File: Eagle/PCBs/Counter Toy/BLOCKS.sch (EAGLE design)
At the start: 6 parts, among them U1 MC74HC1G14DTT1G

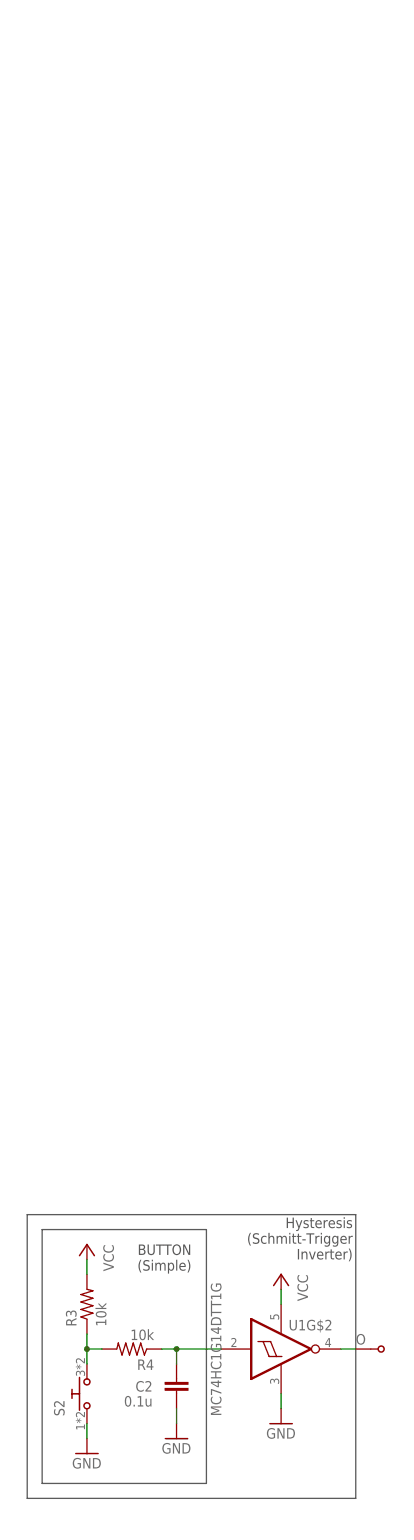
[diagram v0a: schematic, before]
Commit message: Better DFF
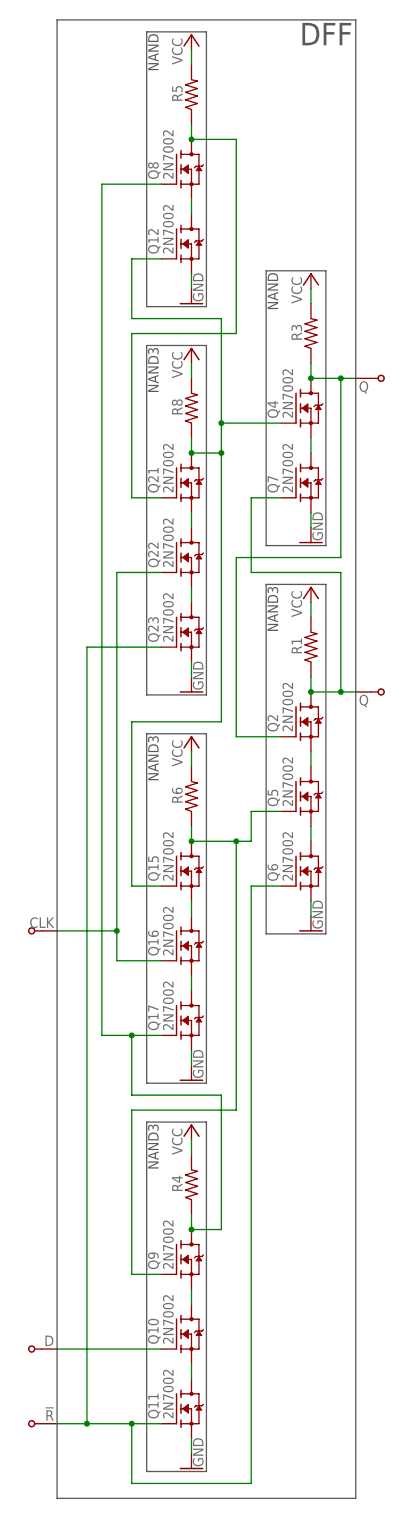
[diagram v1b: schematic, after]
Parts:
- removed C2: 0.1u, ellajameson-core:CAP0603
- removed O: TPPAD6, ellajameson-core:TPPAD6
- removed S2: (no value), ellajameson-core:SWITCH-NO-MOMPTS815SJM250SMTRLFS
- removed U1: MC74HC1G14DTT1G, ellajameson-core:MC74HC1G14DTT1G
- added !Q, !R, CLK, D, Q: TPPAD6, ellajameson-core:TPPAD6
- added Q10, Q11, Q12, Q15, Q16, Q17, Q2, Q21, Q22, Q23, Q4, Q5, Q6, Q7, Q8, Q9: 2N7002, ellajameson-core:2N7002
- added R1, R5, R6, R8: (no value), ellajameson-core:RES0603
- R3, R4: value 10k -> (none)
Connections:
- removed net N$1: O.S, U1G$2.O
- removed net N$3: R3.1, R4.2, S2.S
- new net N$10: Q2.S, Q5.D
- new net N$12: Q5.S, Q6.D
- new net N$14: Q4.S, Q7.D
- new net N$16: Q21.G, Q8.D, R5.1
- new net N$18: Q17.G, Q8.G, Q9.D, R4.1
- new net N$19: D.S, Q10.G
- new net N$20: Q10.D, Q9.S
- new net N$22: Q10.S, Q11.D
- new net N$24: Q12.D, Q8.S
- new net N$31: CLK.S, Q16.G, Q22.G
- new net N$32: Q15.S, Q16.D
- new net N$34: Q16.S, Q17.D
- new net N$44: Q21.S, Q22.D
- new net N$45: !R.S, Q11.G, Q23.G, Q6.G
- new net N$46: Q22.S, Q23.D
- new net N$7: Q12.G, Q15.G, Q21.D, Q4.G, R8.1
- new net N$8: Q.S, Q2.G, Q4.D, R3.1
- new net N$9: Q15.D, Q5.G, Q9.G, R6.1
- net GND: now also Q11.S, Q12.S, Q17.S, Q23.S, Q6.S, Q7.S; no longer C2.2, S2.P, U1G$1.V-
- net N$4: now also !Q.S, Q2.D, Q7.G, R1.1; no longer C2.1, R4.1, U1G$2.I
- net VCC: now also R1.2, R4.2, R5.2, R6.2, R8.2; no longer U1G$1.V+
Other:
- note added: "DFF"
- note added: "NAND"
- note added: "NAND3"
- note removed: "BUTTON (Simple)"
- note removed: "Hysteresis (Schmitt-Trigger Inverter)"
- moved on the sheet: R3, R4

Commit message: Testing open collector setup
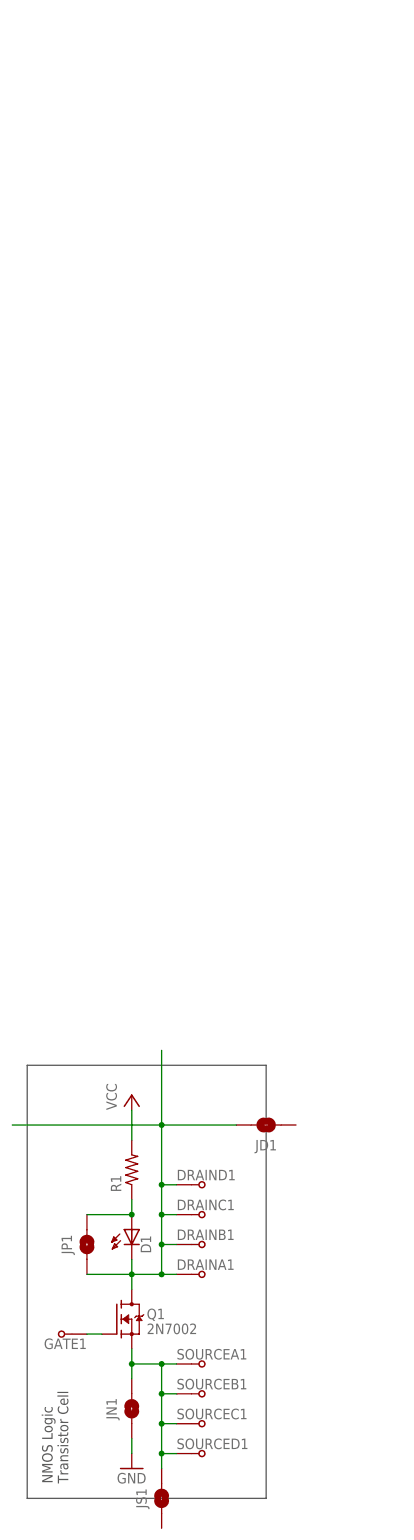
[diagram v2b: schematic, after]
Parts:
- removed !Q, !R, CLK, D, Q: TPPAD6, ellajameson-core:TPPAD6
- removed Q10, Q11, Q12, Q15, Q16, Q17, Q2, Q21, Q22, Q23, Q4, Q5, Q6, Q7, Q8, Q9: 2N7002, ellajameson-core:2N7002
- removed R3, R4, R5, R6, R8: (no value), ellajameson-core:RES0603
- added D1: (no value), ellajameson-core:LED0603
- added DRAINA1, DRAINB1, DRAINC1, DRAIND1, GATE1, SOURCEA1, SOURCEB1, SOURCEC1, SOURCED1: TPWIRE, ellajameson-core:TPWIRE
- added JD1, JN1, JP1, JS1: SJ_NO, ellajameson-core:SJ_NO
- added Q1: 2N7002, ellajameson-core:2N7002
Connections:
- removed net N$10: Q2.S, Q5.D
- removed net N$12: Q5.S, Q6.D
- removed net N$14: Q4.S, Q7.D
- removed net N$16: Q21.G, Q8.D, R5.1
- removed net N$18: Q17.G, Q8.G, Q9.D, R4.1
- removed net N$19: D.S, Q10.G
- removed net N$20: Q10.D, Q9.S
- removed net N$22: Q10.S, Q11.D
- removed net N$24: Q12.D, Q8.S
- removed net N$31: CLK.S, Q16.G, Q22.G
- removed net N$32: Q15.S, Q16.D
- removed net N$34: Q16.S, Q17.D
- removed net N$4: !Q.S, Q2.D, Q7.G, R1.1
- removed net N$44: Q21.S, Q22.D
- removed net N$45: !R.S, Q11.G, Q23.G, Q6.G
- removed net N$46: Q22.S, Q23.D
- removed net N$9: Q15.D, Q5.G, Q9.G, R6.1
- new net N$5: D1.A, JP1.2, R1.1
- new net N$6: D1.K, DRAINA1.S, DRAINB1.S, DRAINC1.S, DRAIND1.S, JD1.2, JP1.1, Q1.D
- net GND: now also JN1.1; no longer Q11.S, Q12.S, Q17.S, Q23.S, Q6.S, Q7.S
- net N$7: now also JN1.2, JS1.2, Q1.S, SOURCEA1.S, SOURCEB1.S, SOURCEC1.S, SOURCED1.S; no longer Q12.G, Q15.G, Q21.D, Q4.G, R8.1
- net N$8: now also GATE1.S, Q1.G; no longer Q.S, Q2.G, Q4.D, R3.1
- net VCC: no longer R3.2, R4.2, R5.2, R6.2, R8.2
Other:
- note added: "NMOS Logic Transistor Cell"
- note removed: "DFF"
- note removed: "NAND"
- note removed: "NAND3"
- moved on the sheet: R1
